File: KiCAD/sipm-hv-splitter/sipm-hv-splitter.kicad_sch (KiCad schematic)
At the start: 11 parts, among them J1 Conn_02x18_Odd_Even, J2 Conn_02x17_Odd_Even, U1 ATmega328-M, U14 TPS7A25, U16 TPS7A25

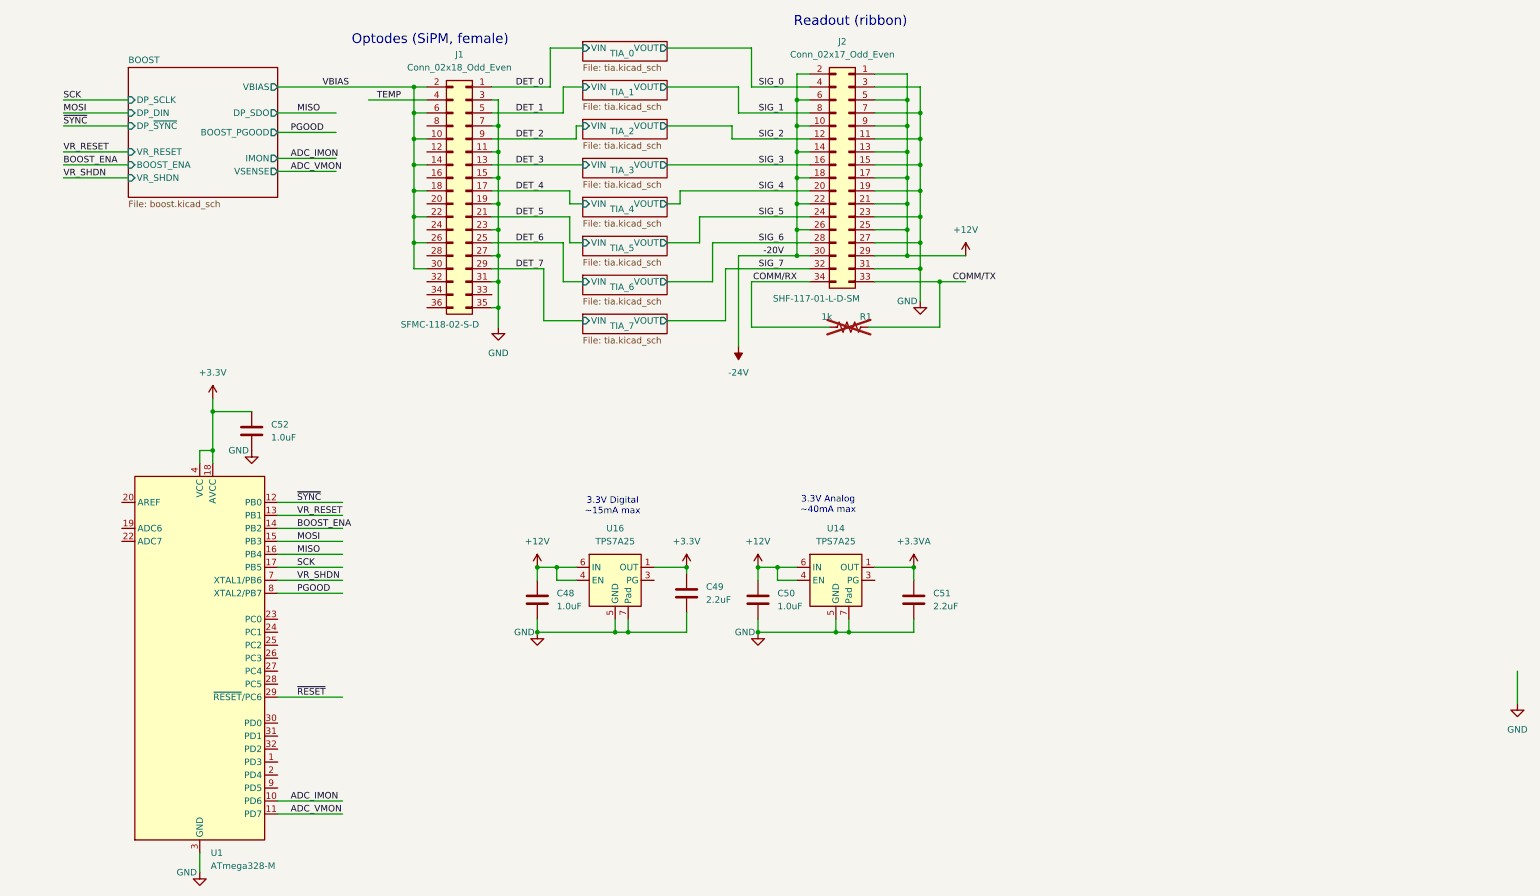
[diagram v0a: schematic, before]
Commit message: add ISP
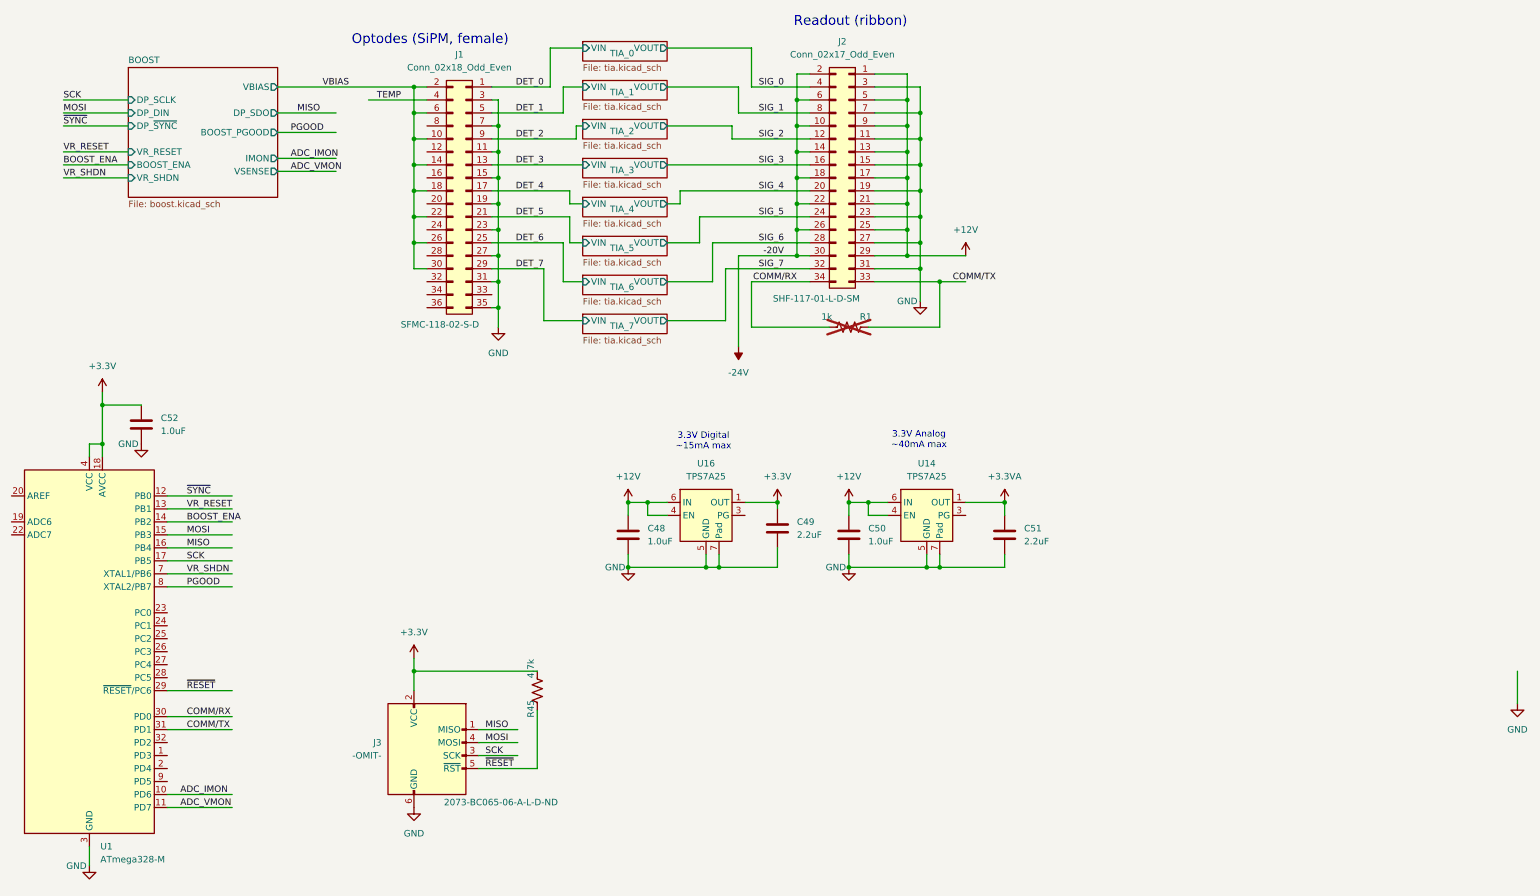
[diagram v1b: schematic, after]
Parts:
- added J3: -OMIT-, Connector_PinHeader_1.00mm:PinHeader_1x06_P1.00mm_Vertical, symbol Connector:AVR-ISP-6
- added R45: 4.7k, Resistor_SMD:R_0603_1608Metric_Pad0.98x0.95mm_HandSolder, symbol Device:R_US
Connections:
- net +3.3V: now also J3.2 (VCC), R45.2
- net COMM/RX: now also U1.30 (PD0)
- net COMM/TX: now also U1.31 (PD1)
- net GND: now also J3.6 (GND)
- net MISO: now also J3.1 (MISO)
- net MOSI: now also J3.4 (MOSI)
- net SCK: now also J3.3 (SCK)
- net ~{RESET}: now also J3.5 (~{RST}), R45.1
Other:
- moved on the sheet: C48, C49, C50, C51, C52, U1, U14, U16
